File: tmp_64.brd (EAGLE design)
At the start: 31.8 x 169.4 mm, 0 parts

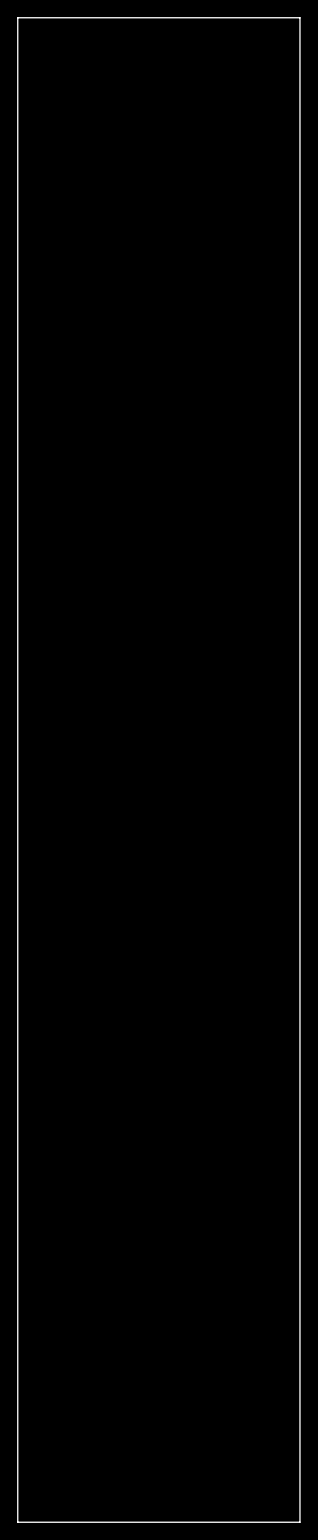
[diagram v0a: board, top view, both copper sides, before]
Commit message: union signal
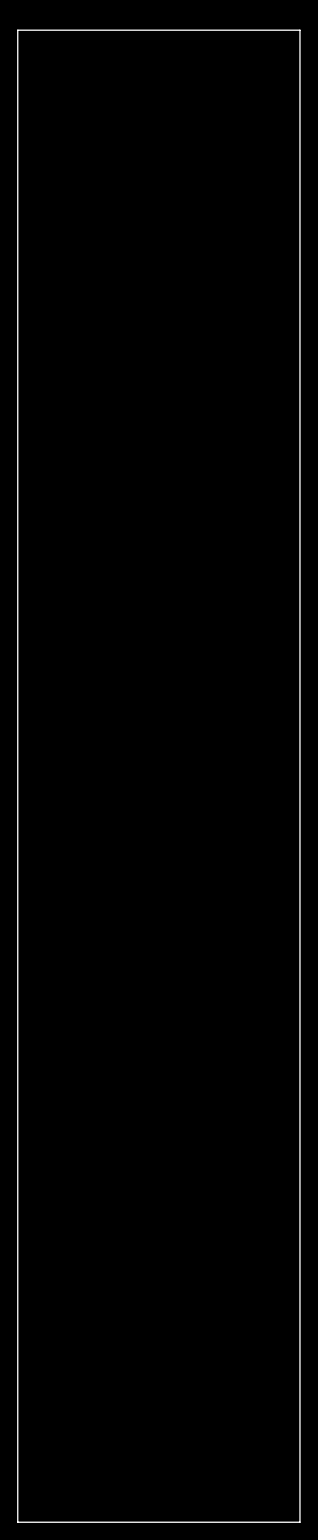
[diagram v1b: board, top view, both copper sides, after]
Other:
- board size 31.8 x 169.4 mm -> 31.8 x 168 mm
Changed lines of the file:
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@@
 <plain>
 <wire x1="0" y1="0" x2="31.78" y2="0" width="0" layer="20"/>
-<wire x1="31.78" y1="0" x2="31.78" y2="169.42" width="0" layer="20"/>
-<wire x1="31.78" y1="169.42" x2="0" y2="169.42" width="0" layer="20"/>
-<wire x1="0" y1="169.42" x2="0" y2="0" width="0" layer="20"/>
+<wire x1="31.78" y1="0" x2="31.78" y2="168.02" width="0" layer="20"/>
+<wire x1="31.78" y1="168.02" x2="0" y2="168.02" width="0" layer="20"/>
+<wire x1="0" y1="168.02" x2="0" y2="0" width="0" layer="20"/>
 </plain>
 <attributes>
@@
 </class>
 </classes>
-<designrules name="default">
+<designrules name="default *">
 <description language="de">&lt;b&gt;EAGLE Design Rules&lt;/b&gt;
 &lt;p&gt;
@@
 <param name="mtCopper" value="0.035mm 0.035mm 0.035mm 0.035mm 0.035mm 0.035mm 0.035mm 0.035mm 0.035mm 0.035mm 0.035mm 0.035mm 0.035mm 0.035mm 0.035mm 0.035mm"/>
 <param name="mtIsolate" value="1.5mm 0.15mm 0.2mm 0.15mm 0.2mm 0.15mm 0.2mm 0.15mm 0.2mm 0.15mm 0.2mm 0.15mm 0.2mm 0.15mm 0.2mm"/>
-<param name="mdWireWire" value="8mil"/>
-<param name="mdWirePad" value="8mil"/>
+<param name="mdWireWire" value="12mil"/>
+<param name="mdWirePad" value="10mil"/>
 <param name="mdWireVia" value="8mil"/>
 <param name="mdPadPad" value="8mil"/>
